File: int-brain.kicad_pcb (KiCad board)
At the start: 2 copper layers, 117.4 x 66.6 mm, 62 parts, among them J1 PWR, J10 Left, J11 Right, J2 UART0, J3 I2C0, J4 PWR, J5 1MA, J6 1MB, J7 2MA, J8 2MB, J9 MPU9250, U1 L298N, U2 ESP32-DevKitC, U3 L298N, U4 LM2576HVT-5

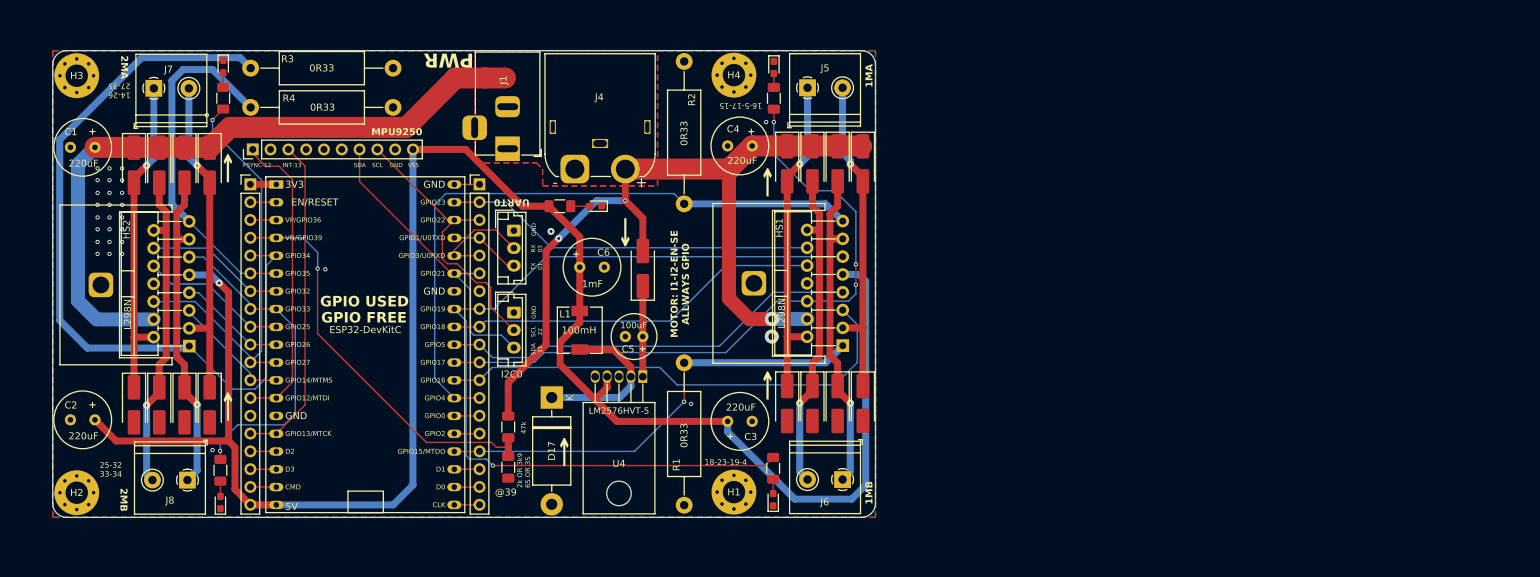
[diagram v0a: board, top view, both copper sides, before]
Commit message: done placement
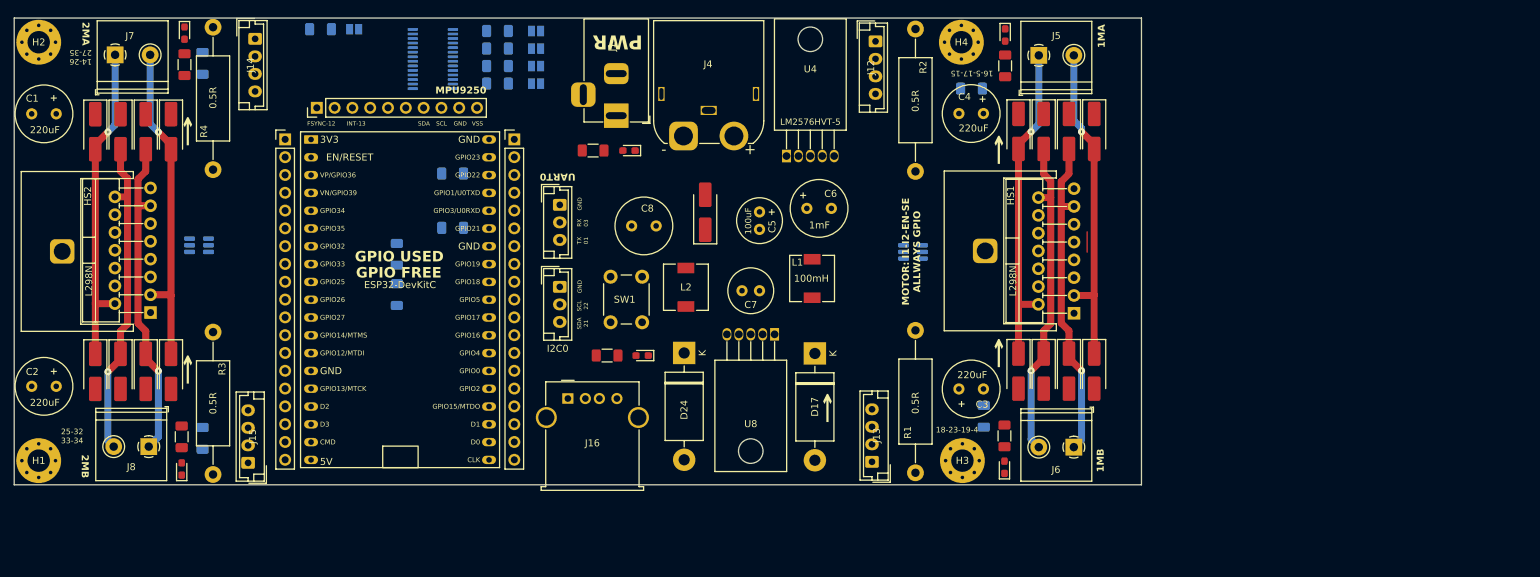
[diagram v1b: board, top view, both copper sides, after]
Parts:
- added C7: 100uF, Capacitor_THT:C_Radial_D6.3mm_H11.0mm_P2.50mm, F.Cu at (161.2, 82.7)
- added C8: 1mF, Capacitor_THT:C_Radial_D8.0mm_H11.5mm_P3.50mm, F.Cu at (143.0, 73.4)
- added D24: 1N5822, Diode_THT:D_DO-201AD_P15.24mm_Horizontal, F.Cu at (150.5, 91.5)
- added D25: PWR, LED_SMD:LED_0603_1608Metric_Pad1.05x0.95mm_HandSolder, F.Cu at (144.5, 91.9)
- added J12: 1MA_ENC, Connector_JST:JST_EH_B4B-EH-A_1x04_P2.50mm_Vertical, F.Cu at (177.8, 47.1)
- added J13: 1MB_ENC, Connector_JST:JST_EH_B4B-EH-A_1x04_P2.50mm_Vertical, F.Cu at (177.3, 107.1)
- added J14: 2MA_ENC, Connector_JST:JST_EH_B4B-EH-A_1x04_P2.50mm_Vertical, F.Cu at (89.3, 46.7)
- added J15: 2MB_ENC, Connector_JST:JST_EH_B4B-EH-A_1x04_P2.50mm_Vertical, F.Cu at (88.3, 107.2)
- added J16: USB_A, Connector_USB:USB_A_Molex_67643_Horizontal, F.Cu at (133.9, 98.0)
- added JP1: SolderJumper_2_Open, Jumper:SolderJumper-2_P1.3mm_Open_Pad1.0x1.5mm, B.Cu at (129.4, 45.6)
- added JP2: SolderJumper_2_Open, Jumper:SolderJumper-2_P1.3mm_Open_Pad1.0x1.5mm, B.Cu at (129.4, 48.1)
- added JP3: SolderJumper_2_Open, Jumper:SolderJumper-2_P1.3mm_Open_Pad1.0x1.5mm, B.Cu at (129.4, 50.6)
- added JP4: SolderJumper_2_Open, Jumper:SolderJumper-2_P1.3mm_Open_Pad1.0x1.5mm, B.Cu at (129.4, 53.1)
- added JP5: SolderJumper_2_Open, Jumper:SolderJumper-2_P1.3mm_Open_Pad1.0x1.5mm, B.Cu at (103.4, 45.4)
- added L2: 100mH, Inductor_SMD:L_6.3x6.3_H3, F.Cu at (150.8, 82.2)
- added R12: 10k, Resistor_SMD:R_1206_3216Metric_Pad1.30x1.75mm_HandSolder, B.Cu at (191.5, 53.8)
- added R13: 10k, Resistor_SMD:R_1206_3216Metric_Pad1.30x1.75mm_HandSolder, B.Cu at (81.8, 50.2)
- added R14: 10k, Resistor_SMD:R_1206_3216Metric_Pad1.30x1.75mm_HandSolder, B.Cu at (193.2, 100.6)
- added R15: 10k, Resistor_SMD:R_1206_3216Metric_Pad1.30x1.75mm_HandSolder, B.Cu at (81.8, 103.7)
- added R16: 4.7k, Resistor_SMD:R_1206_3216Metric_Pad1.30x1.75mm_HandSolder, B.Cu at (117.5, 65.9)
- added R17: 4.7k, Resistor_SMD:R_1206_3216Metric_Pad1.30x1.75mm_HandSolder, B.Cu at (117.5, 73.7)
- added R18: 10k, Resistor_SMD:R_1206_3216Metric_Pad1.30x1.75mm_HandSolder, B.Cu at (123.9, 45.6)
- added R19: 10k, Resistor_SMD:R_1206_3216Metric_Pad1.30x1.75mm_HandSolder, B.Cu at (123.9, 48.1)
- added R20: 10k, Resistor_SMD:R_1206_3216Metric_Pad1.30x1.75mm_HandSolder, B.Cu at (123.9, 50.6)
- added R21: 10k, Resistor_SMD:R_1206_3216Metric_Pad1.30x1.75mm_HandSolder, B.Cu at (123.9, 53.1)
- added R22: 10k, Resistor_SMD:R_1206_3216Metric_Pad1.30x1.75mm_HandSolder, B.Cu at (98.6, 45.4)
- added R23: 470R, Resistor_SMD:R_1206_3216Metric_Pad1.30x1.75mm_HandSolder, F.Cu at (139.5, 91.9)
- added SW1: SW_Push, Button_Switch_THT:SW_PUSH_6mm_H5mm, F.Cu at (144.5, 80.7)
- added U5: 74LVC2G04, Package_TO_SOT_SMD:SOT-23-6_Handsoldering, B.Cu at (183.2, 77.1)
- added U6: 74LVC2G04, Package_TO_SOT_SMD:SOT-23-6_Handsoldering, B.Cu at (81.3, 76.2)
- added U7: PCA9635, Package_SO:TSSOP-28_4.4x9.7mm_P0.65mm, B.Cu at (114.6, 49.6)
- added U8: LM2576HVT-5, Package_TO_SOT_THT:TO-220-5_Horizontal_TabDown, F.Cu at (163.4, 88.9)
- R1, R2, R3, R4: value 0R33 -> 0.5R
- R10: moved to B.Cu
- R11: value 3.9k -> 10k; moved to B.Cu
- moved H3 137.8 mm to (190.2, 106.9)
- moved H1 99.3 mm to (58.4, 106.9)
- moved H2 64.5 mm to (58.4, 47.2)
- moved D17 38.1 mm to (169.2, 91.6)
- moved R3 38.0 mm to (83.3, 88.6), turned to -90 degrees
- moved U4 37.6 mm to (165.1, 63.4), turned to 0 degrees
- moved L1 34.0 mm to (168.8, 80.9)
- moved C6 33.5 mm to (168.0, 70.9)
- moved C3 33.3 mm to (193.2, 96.7)
- moved C4 33.3 mm to (189.7, 57.4)
- moved D1 33.3 mm to (198.2, 59.9)
- moved D18 33.3 mm to (196.3, 46.2)
- moved D19 33.3 mm to (196.2, 107.8)
- moved D2 33.3 mm to (198.2, 94.1)
- moved D3 33.3 mm to (209.0, 59.9)
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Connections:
- net /BUCK_OUT renamed /BUCK_OUT_1
- net /PWR_LED renamed /PWR_LED_1
- net /VIN_BUCK renamed VIN_BUCK
- J10 pad 10: 2MA2_IN -> /2MA1_ENC
- J10 pad 11: 2MA_EN -> /2MA2_ENC
- J10 pad 12: 2MA1_IN -> /2MB1_ENC
- J10 pad 13: FSYNC -> /2MB2_ENC
- J10 pad 15: INT -> /GPIO13
- J10 pad 3: /GPIO36 -> 2MB_SENSE
- J10 pad 4: VBATT -> 2MA_SENSE
- J10 pad 5: 2MB_SENSE -> 1MB_SENSE
- J10 pad 6: 2MA_SENSE -> 1MA_SENSE
- J10 pad 7: 2MB2_IN -> FSYNC
- J10 pad 8: 2MB_EN -> INT
- J10 pad 9: 2MB1_IN -> VBATT
- J11 pad 10: 1MA2_IN -> /1MB2_ENC
- J11 pad 11: 1MA_EN -> /1MB1_ENC
- J11 pad 12: 1MA1_IN -> /GPIO16
- J11 pad 13: 1MB_SENSE -> M_OE
- J11 pad 16: 1MA_SENSE -> /GPIO15
- J11 pad 2: 1MB2_IN -> /GPIO23
- J11 pad 8: 1MB_EN -> /1MA1_ENC
- J11 pad 9: 1MB1_IN -> /1MA2_ENC
- R5 pad 1: 1MA_EN -> /1MA_EN
- R6 pad 1: 1MB_EN -> /1MB_EN
- R7 pad 1: 2MA_EN -> /2MA_EN
- R8 pad 1: 2MB_EN -> /2MB_EN
- U1 pad 10: 1MB1_IN -> /1MB1_IN
- U1 pad 11: 1MB_EN -> /1MB_EN
- U1 pad 12: 1MB2_IN -> Net-(U1-IN4)
- U1 pad 5: 1MA1_IN -> /1MA1_IN
- U1 pad 6: 1MA_EN -> /1MA_EN
- U1 pad 7: 1MA2_IN -> Net-(U1-IN2)
- U2 pad 10: 2MA2_IN -> /2MA1_ENC
- U2 pad 11: 2MA_EN -> /2MA2_ENC
- U2 pad 12: 2MA1_IN -> /2MB1_ENC
- U2 pad 13: FSYNC -> /2MB2_ENC
- U2 pad 15: INT -> /GPIO13
- U2 pad 23: 1MA_SENSE -> /GPIO15
- U2 pad 26: 1MB_SENSE -> M_OE
- U2 pad 27: 1MA1_IN -> /GPIO16
- U2 pad 28: 1MA_EN -> /1MB1_ENC
- U2 pad 29: 1MA2_IN -> /1MB2_ENC
- U2 pad 3: /GPIO36 -> 2MB_SENSE
- U2 pad 30: 1MB1_IN -> /1MA2_ENC
- U2 pad 31: 1MB_EN -> /1MA1_ENC
- U2 pad 37: 1MB2_IN -> /GPIO23
- U2 pad 4: VBATT -> 2MA_SENSE
- U2 pad 5: 2MB_SENSE -> 1MB_SENSE
- U2 pad 6: 2MA_SENSE -> 1MA_SENSE
- U2 pad 7: 2MB2_IN -> FSYNC
- U2 pad 8: 2MB_EN -> INT
- U2 pad 9: 2MB1_IN -> VBATT
- U3 pad 10: 2MB1_IN -> /2MB1_IN
- U3 pad 11: 2MB_EN -> /2MB_EN
- U3 pad 12: 2MB2_IN -> Net-(U3-IN4)
- U3 pad 5: 2MA1_IN -> /2MA1_IN
- U3 pad 6: 2MA_EN -> /2MA_EN
- U3 pad 7: 2MA2_IN -> Net-(U3-IN2)
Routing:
- net VSS: track 269.2 -> 0.00 mm, vias 1 -> 0
- net VS: track 216.3 -> 0.00 mm, vias 3 -> 0
- net 1MB_EN: track 125.0 -> 0.00 mm, vias 1 -> 0
- net 2MB_SENSE: track 114.7 -> 0.40 mm
- net 1MA_EN: track 94.6 -> 0.00 mm, vias 3 -> 0
- net 1MB_SENSE: track 92.9 -> 0.00 mm
- net 1MA1_IN: track 69.3 -> 0.00 mm
- net 1MA_SENSE: track 64.9 -> 0.00 mm, vias 1 -> 0
- net 2MA_EN: track 61.9 -> 0.00 mm, vias 1 -> 0
- net 1MA2_IN: track 60.1 -> 0.00 mm
- net VBATT: track 58.6 -> 0.00 mm, vias 1 -> 0
- net 1MB1_IN: track 54.0 -> 0.00 mm
- net 1MB2_IN: track 53.0 -> 0.00 mm
- net 2MA_SENSE: track 50.7 -> 0.00 mm
- net INT: track 47.0 -> 0.00 mm
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- removed copper zone on B.Cu, net GND
- removed copper zone on F.Cu, net GND
- removed copper zone on F.Cu, net VS
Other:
- board size 117.4 x 66.6 mm -> 160.8 x 66.6 mm

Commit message: done placement again
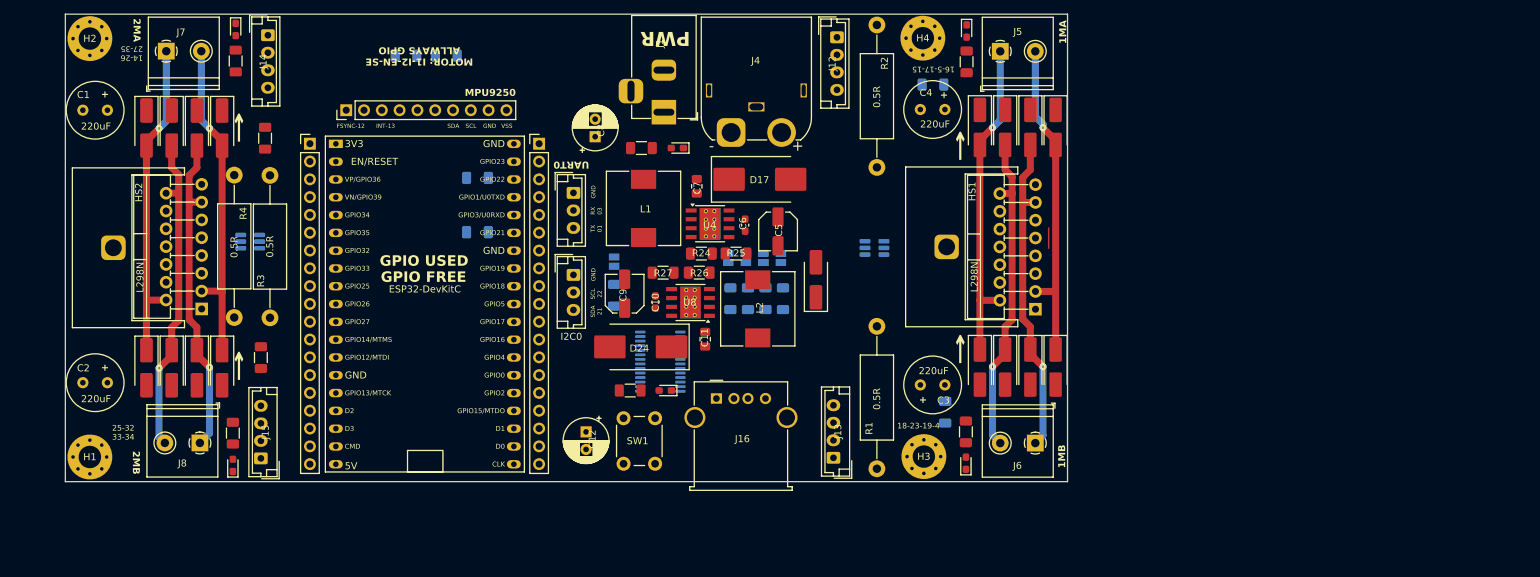
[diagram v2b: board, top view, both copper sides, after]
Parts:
- added C10: 4.7uF, Capacitor_SMD:C_0603_1608Metric_Pad1.08x0.95mm_HandSolder, F.Cu at (146.4, 84.3)
- added C11: 10nF, Capacitor_SMD:C_0805_2012Metric_Pad1.18x1.45mm_HandSolder, F.Cu at (153.5, 89.6)
- added C12: 220uF, Capacitor_THT:CP_Radial_D6.3mm_P2.50mm, F.Cu at (136.5, 102.8)
- added C9: 4.7uF, Capacitor_SMD:C_Elec_5x5.8, F.Cu at (142.0, 83.1)
- added R24: 10k, Resistor_SMD:R_1206_3216Metric_Pad1.30x1.75mm_HandSolder, F.Cu at (152.9, 77.4)
- added R25: 3.24k, Resistor_SMD:R_1206_3216Metric_Pad1.30x1.75mm_HandSolder, F.Cu at (157.9, 77.4)
- added R26: 10k, Resistor_SMD:R_1206_3216Metric_Pad1.30x1.75mm_HandSolder, F.Cu at (152.7, 80.1)
- added R27: 3.24k, Resistor_SMD:R_1206_3216Metric_Pad1.30x1.75mm_HandSolder, F.Cu at (147.5, 80.1)
- C5: value 100uF -> 4.7uF; footprint Capacitor_THT:C_Radial_D6.3mm_H11.0mm_P2.50mm -> Capacitor_SMD:C_Elec_5x5.8
- C6: value 1mF -> 4.7uF; footprint Capacitor_THT:C_Radial_D8.0mm_H11.5mm_P3.50mm -> Capacitor_SMD:C_0603_1608Metric_Pad1.08x0.95mm_HandSolder
- C7: value 100uF -> 10nF; footprint Capacitor_THT:C_Radial_D6.3mm_H11.0mm_P2.50mm -> Capacitor_SMD:C_0805_2012Metric_Pad1.18x1.45mm_HandSolder
- C8: value 1mF -> 220uF; footprint Capacitor_THT:C_Radial_D8.0mm_H11.5mm_P3.50mm -> Capacitor_THT:CP_Radial_D6.3mm_P2.50mm
- D17, D24: value 1N5822 -> B340; footprint Diode_THT:D_DO-201AD_P15.24mm_Horizontal -> Diode_SMD:D_SMC_Handsoldering
- L1, L2: value 100mH -> 22uH; footprint Inductor_SMD:L_6.3x6.3_H3 -> Inductor_SMD:L_10.4x10.4_H4.8
- R13, R15: moved to F.Cu
- U4, U8: value LM2576HVT-5 -> TPS5430DDA; footprint Package_TO_SOT_THT:TO-220-5_Horizontal_TabDown -> Package_SO:TI_SO-PowerPAD-8_ThermalVias
- moved R22 56.5 mm to (140.5, 83.3), turned to 90 degrees
- moved U7 54.0 mm to (147.1, 92.8)
- moved R21 51.0 mm to (164.6, 83.8), turned to -90 degrees
- moved R20 50.6 mm to (162.1, 83.8), turned to -90 degrees
- moved R18 50.6 mm to (157.1, 83.8), turned to -90 degrees
- moved R19 50.5 mm to (159.6, 83.8), turned to -90 degrees
- moved JP5 49.8 mm to (140.5, 78.5), turned to -90 degrees
- moved JP4 42.9 mm to (164.3, 78.0), turned to 90 degrees
- moved JP3 42.4 mm to (161.8, 78.0), turned to -90 degrees
- moved JP1 42.4 mm to (156.8, 78.0), turned to -90 degrees
- moved JP2 42.3 mm to (159.3, 78.0), turned to -90 degrees
- moved R11 34.1 mm to (110.8, 49.1), turned to 180 degrees
- moved R10 29.2 mm to (116.5, 49.1), turned to 180 degrees
- moved D17 26.1 mm to (161.3, 66.8), turned to 0 degrees
- moved L1 26.0 mm to (144.7, 70.9), turned to -90 degrees
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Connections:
- C5 pad 1: VIN_BUCK -> BUCK_VS
- C6 pad 1: VSS -> BUCK_VS
- C7 pad 1: /SBC_VIN_BUCK -> Net-(U4-BOOT)
- C7 pad 2: GND -> /buck1/BUCK_OUT
- C8 pad 1: /SBC_VSS -> VSS
- D17 pad 1: /BUCK_OUT_1 -> /buck1/BUCK_OUT
- D23 pad 1: VIN_BUCK -> BUCK_VS
- D24 pad 1: /BUCK_OUT_2 -> /buck2/BUCK_OUT
- J16 pad 1: /SBC_VSS -> /buck2/VOUT
- L1 pad 1: /BUCK_OUT_1 -> /buck1/BUCK_OUT
- L2 pad 1: /BUCK_OUT_2 -> /buck2/BUCK_OUT
- L2 pad 2: /SBC_VSS -> /buck2/VOUT
- R23 pad 1: /SBC_VSS -> /buck2/VOUT
- SW1 pad 1: VIN_BUCK -> BUCK_VS
- SW1 pad 2: /SBC_VIN_BUCK -> /buck2/BUCK_VIN
- U4 pad 1: VIN_BUCK -> Net-(U4-BOOT)
- U4 pad 2: /BUCK_OUT_1 -> unconnected-(U4-NC-Pad2)
- U4 pad 3: GND -> unconnected-(U4-NC-Pad3)
- U4 pad 4: VSS -> /buck1/BUCK_VSENSE
- U4 pad 5: GND -> unconnected-(U4-EN-Pad5)
- U8 pad 1: /SBC_VIN_BUCK -> Net-(U8-BOOT)
- U8 pad 2: /BUCK_OUT_2 -> unconnected-(U8-NC-Pad2)
- U8 pad 3: GND -> unconnected-(U8-NC-Pad3)
- U8 pad 4: /SBC_VSS -> /buck2/BUCK_VSENSE
- U8 pad 5: GND -> unconnected-(U8-EN-Pad5)
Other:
- board size 160.8 x 66.6 mm -> 143 x 66.7 mm

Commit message: done!?!?!
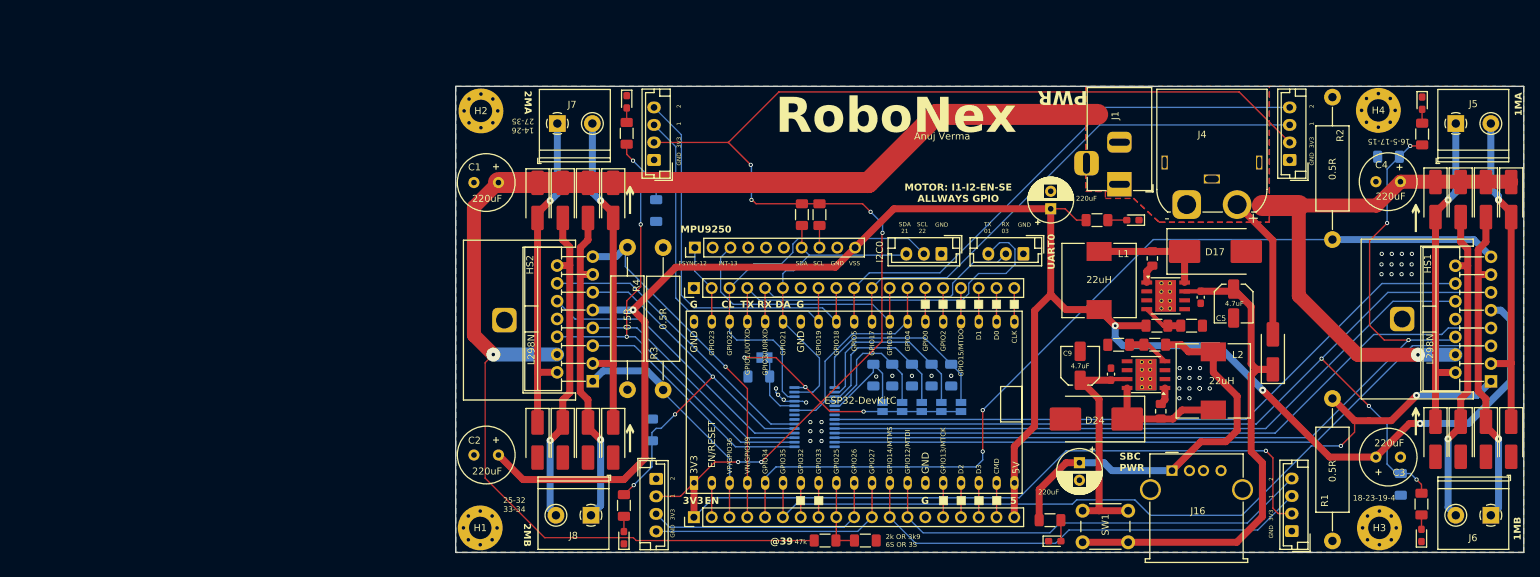
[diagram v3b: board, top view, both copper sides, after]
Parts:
- removed U5, U6: 74LVC2G04, Package_TO_SOT_SMD:SOT-23-6_Handsoldering
- added JP0: A0, Jumper:SolderJumper-2_P1.3mm_Open_Pad1.0x1.5mm, B.Cu at (190.0, 99.2)
- added R28: 10k, Resistor_SMD:R_1206_3216Metric_Pad1.30x1.75mm_HandSolder, B.Cu at (188.6, 94.7)
- JP1: value SolderJumper_2_Open -> A1
- JP2: value SolderJumper_2_Open -> A2
- JP3: value SolderJumper_2_Open -> A3
- JP4: value SolderJumper_2_Open -> A4
- JP5: value SolderJumper_2_Open -> A5
- R10, R11, R16, R17: moved to F.Cu
- R13, R15: moved to B.Cu
- moved J15 147.5 mm to (237.2, 117.0)
- moved R11 95.3 mm to (176.3, 118.3), turned to 0 degrees
- moved R10 87.8 mm to (170.6, 118.3), turned to 0 degrees
- moved J14 84.1 mm to (146.5, 109.5)
- moved J13 77.7 mm to (236.9, 64.0)
- moved J10 76.4 mm to (151.9, 115.0), turned to 90 degrees
- moved C12 70.5 mm to (206.9, 107.2)
- moved U2 70.4 mm to (151.9, 110.1), turned to 90 degrees
- moved SW1 69.8 mm to (213.8, 118.5), turned to 180 degrees
- moved D23 66.0 mm to (234.5, 91.4)
- moved J5 65.8 mm to (260.6, 58.8)
- moved J6 65.8 mm to (265.6, 114.7)
- moved C3 65.8 mm to (252.7, 106.4)
- moved C4 65.8 mm to (249.2, 67.1)
- moved D1 65.8 mm to (257.7, 69.7)
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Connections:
- J10 pad 10: /2MA1_ENC -> /2MB1_ENC
- J10 pad 11: /2MA2_ENC -> /2MB2_ENC
- J10 pad 12: /2MB1_ENC -> /1MB1_ENC
- J10 pad 13: /2MB2_ENC -> /1MB2_ENC
- J10 pad 7: FSYNC -> /GPIO32
- J10 pad 8: INT -> /GPIO33
- J11 pad 10: /1MB2_ENC -> /1MA2_ENC
- J11 pad 11: /1MB1_ENC -> /1MA1_ENC
- J11 pad 12: /GPIO16 -> INT
- J11 pad 2: /GPIO23 -> FSYNC
- J11 pad 8: /1MA1_ENC -> /2MA1_ENC
- J11 pad 9: /1MA2_ENC -> /2MA2_ENC
- J12 pad 3: /1MA1_ENC -> /2MA1_ENC
- J12 pad 4: /1MA2_ENC -> /2MA2_ENC
- J13 pad 3: /1MB1_ENC -> /1MA1_ENC
- J13 pad 4: /1MB2_ENC -> /1MA2_ENC
- J14 pad 3: /2MA1_ENC -> /2MB1_ENC
- J14 pad 4: /2MA2_ENC -> /2MB2_ENC
- J15 pad 3: /2MB1_ENC -> /1MB1_ENC
- J15 pad 4: /2MB2_ENC -> /1MB2_ENC
- U1 pad 12: Net-(U1-IN4) -> /1MB2_IN
- U1 pad 7: Net-(U1-IN2) -> /1MA2_IN
- U2 pad 10: /2MA1_ENC -> /2MB1_ENC
- U2 pad 11: /2MA2_ENC -> /2MB2_ENC
- U2 pad 12: /2MB1_ENC -> /1MB1_ENC
- U2 pad 13: /2MB2_ENC -> /1MB2_ENC
- U2 pad 27: /GPIO16 -> INT
- U2 pad 28: /1MB1_ENC -> /1MA1_ENC
- U2 pad 29: /1MB2_ENC -> /1MA2_ENC
- U2 pad 30: /1MA2_ENC -> /2MA2_ENC
- U2 pad 31: /1MA1_ENC -> /2MA1_ENC
- U2 pad 37: /GPIO23 -> FSYNC
- U2 pad 7: FSYNC -> /GPIO32
- U2 pad 8: INT -> /GPIO33
- U3 pad 12: Net-(U3-IN4) -> /2MB2_IN
- U3 pad 7: Net-(U3-IN2) -> /2MA2_IN
- U7 pad 1: +3.3V -> /PCA_A0
- U7 pad 10: /1MB_EN -> /1MB1_IN
- U7 pad 11: /1MB1_IN -> /1MA2_IN
- U7 pad 17: /2MB1_IN -> /2MA2_IN
- U7 pad 18: /2MB_EN -> /2MB1_IN
- U7 pad 19: unconnected-(U7-LED12-Pad19) -> /2MB_EN
- U7 pad 20: unconnected-(U7-LED13-Pad20) -> /2MB2_IN
- U7 pad 8: unconnected-(U7-LED2-Pad8) -> /1MB2_IN
- U7 pad 9: unconnected-(U7-LED3-Pad9) -> /1MB_EN
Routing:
- net +3.3V: track 0.00 -> 324.5 mm, vias 0 -> 10
- net VS: track 0.00 -> 290.8 mm, vias 0 -> 2
- net VSS: track 0.00 -> 266.0 mm, vias 0 -> 4
- net /1MA_EN: track 0.00 -> 130.7 mm, vias 0 -> 3
- net 1MB_SENSE: track 0.00 -> 128.5 mm, vias 0 -> 2
- net /1MB_EN: track 0.00 -> 127.7 mm, vias 0 -> 3
- net 1MA_SENSE: track 0.00 -> 121.2 mm, vias 0 -> 2
- net /1MA2_IN: track 0.00 -> 99.9 mm
- net /1MA1_IN: track 0.00 -> 99.4 mm
- net /1MB2_IN: track 0.00 -> 96.6 mm
- net /1MB1_IN: track 0.00 -> 96.1 mm
- net /1MA2_ENC: track 0.00 -> 77.6 mm
- net /2MA_EN: track 0.00 -> 74.1 mm, vias 0 -> 3
- net /1MA1_ENC: track 0.00 -> 74.1 mm
- net BUCK_VS: track 0.00 -> 73.7 mm
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- added copper zone on B.Cu, net GND
- added copper zone on F.Cu, net GND
- added copper zone on F.Cu, net VS
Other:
- board size 143 x 66.7 mm -> 152.4 x 66.5 mm
- board text added: "1"
- board text added: "2"
- board text added: "3V3"
- board text added: "5"
- board text added: "Anuj Verma"
- board text added: "CL"
- board text added: "DA"
- board text added: "EN"
- board text added: "G"
- board text added: "RX"
- board text added: "RoboNex"
- board text added: "SBC PWR"
- board text added: "TX"
- board text removed: "GPIO FREE"
- board text removed: "GPIO USED"
